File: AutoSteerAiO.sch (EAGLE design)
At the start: 82 parts, among them IC2 MMA8452Q, J4 CONNECTOR 1x5 PINS, K4 CB1A-P-12V

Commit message: Add files via upload
silkscreen
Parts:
- +5V, +5V1, GND33, GND34: MPN HEF4093BT,653 -> (none); OC_NEWARK 70R5288 -> unknown
- U$3: MPN (none) -> ATSAMD10C13A-SSNT; OC_NEWARK (none) -> 90Y6375
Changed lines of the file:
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@@
 <part name="+5V" library="wirepad" library_urn="urn:adsk.eagle:library:412" deviceset="2,15/1,0" device="" package3d_urn="urn:adsk.eagle:package:30831/1">
 <attribute name="MF" value=""/>
-<attribute name="MPN" value="HEF4093BT,653"/>
-<attribute name="OC_NEWARK" value="70R5288"/>
+<attribute name="MPN" value=""/>
+<attribute name="OC_NEWARK" value="unknown"/>
 </part>
 <part name="+5V1" library="wirepad" library_urn="urn:adsk.eagle:library:412" deviceset="2,15/1,0" device="" package3d_urn="urn:adsk.eagle:package:30831/1">
 <attribute name="MF" value=""/>
-<attribute name="MPN" value="HEF4093BT,653"/>
-<attribute name="OC_NEWARK" value="70R5288"/>
+<attribute name="MPN" value=""/>
+<attribute name="OC_NEWARK" value="unknown"/>
 </part>
 <part name="GND33" library="wirepad" library_urn="urn:adsk.eagle:library:412" deviceset="2,15/1,0" device="" package3d_urn="urn:adsk.eagle:package:30831/1">
 <attribute name="MF" value=""/>
-<attribute name="MPN" value="HEF4093BT,653"/>
-<attribute name="OC_NEWARK" value="70R5288"/>
+<attribute name="MPN" value=""/>
+<attribute name="OC_NEWARK" value="unknown"/>
 </part>
 <part name="GND34" library="wirepad" library_urn="urn:adsk.eagle:library:412" deviceset="2,15/1,0" device="" package3d_urn="urn:adsk.eagle:package:30831/1">
 <attribute name="MF" value=""/>
-<attribute name="MPN" value="HEF4093BT,653"/>
-<attribute name="OC_NEWARK" value="70R5288"/>
+<attribute name="MPN" value=""/>
+<attribute name="OC_NEWARK" value="unknown"/>
 </part>
 <part name="GND25" library="supply1" library_urn="urn:adsk.eagle:library:371" deviceset="GND" device=""/>
@@
 <attribute name="OC_NEWARK" value="unknown"/>
 </part>
-<part name="U$3" library="#Motor Drivers" deviceset="MD10C" device=""/>
+<part name="U$3" library="#Motor Drivers" deviceset="MD10C" device="">
+<attribute name="MF" value=""/>
+<attribute name="MPN" value="ATSAMD10C13A-SSNT"/>
+<attribute name="OC_NEWARK" value="90Y6375"/>
+</part>
 </parts>
 <sheets>
@@
 <attribute name="MPN" x="147.32" y="231.14" size="1.778" layer="96" display="off"/>
 </instance>
-<instance part="U$3" gate="G$1" x="144.78" y="139.7" smashed="yes"/>
+<instance part="U$3" gate="G$1" x="144.78" y="139.7" smashed="yes">
+<attribute name="OC_NEWARK" x="144.78" y="139.7" size="1.778" layer="96" display="off"/>
+<attribute name="MF" x="144.78" y="139.7" size="1.778" layer="96" display="off"/>
+<attribute name="MPN" x="144.78" y="139.7" size="1.778" layer="96" display="off"/>
+</instance>
 </instances>
 <busses>

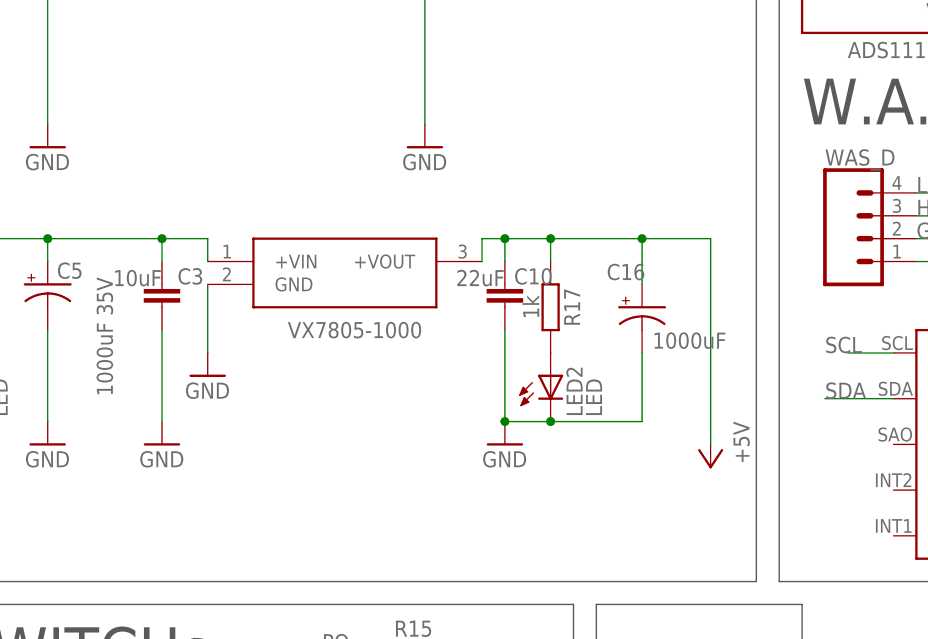
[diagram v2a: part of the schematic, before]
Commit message: Add files via upload
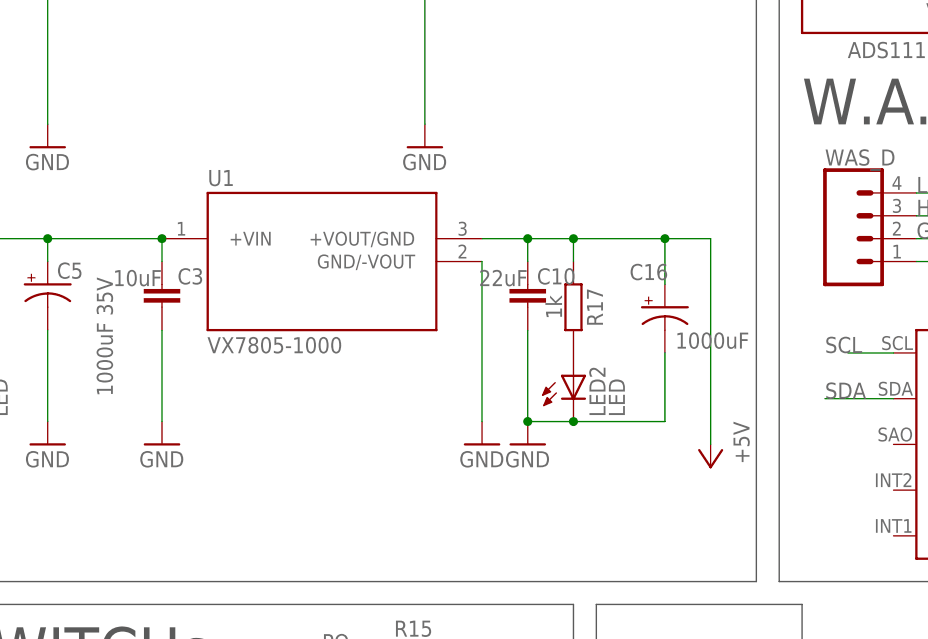
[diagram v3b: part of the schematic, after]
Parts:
- removed PS2: VX7805-1000, #VX7805-500:VX7805-500
- added U1: VX7805-1000, #VX7805-1000:VX7805-1000
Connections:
- net +5V: now also U1.+VOUT/GND; no longer PS2.+VOUT
- net GND: now also U1.GND/-VOUT; no longer PS2.GND
- net N$26: now also U1.+VIN; no longer PS2.+VIN
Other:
- moved on the sheet: C10, C16, LED2, R17

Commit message: Add files via upload
wrong footprint VX7805-1000 it can fit but will come out with PCB
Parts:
- U1: OC_NEWARK (none) -> unknown
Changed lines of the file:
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@@
 <attribute name="OC_NEWARK" value="90Y6375"/>
 </part>
-<part name="U1" library="#VX7805-1000" deviceset="VX7805-1000" device=""/>
+<part name="U1" library="#VX7805-1000" deviceset="VX7805-1000" device="">
+<attribute name="MF" value=""/>
+<attribute name="MPN" value=""/>
+<attribute name="OC_NEWARK" value="unknown"/>
+</part>
 </parts>
 <sheets>
@@
 <attribute name="NAME" x="99.0437" y="244.612709375" size="1.78026875" layer="95"/>
 <attribute name="VALUE" x="99.023" y="226.0304" size="1.78318125" layer="96"/>
+<attribute name="OC_NEWARK" x="111.76" y="236.22" size="1.778" layer="96" display="off"/>
+<attribute name="MPN" x="111.76" y="236.22" size="1.778" layer="96" display="off"/>
 </instance>
 </instances>
